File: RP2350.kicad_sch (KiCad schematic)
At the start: 36 parts, among them SW1 SW_Push, SW2 SW_Push, SW3 SW_Push, U1 RP2350A, U4 AMS1117-3.3, U5 ABM8-272-T3_C20625731

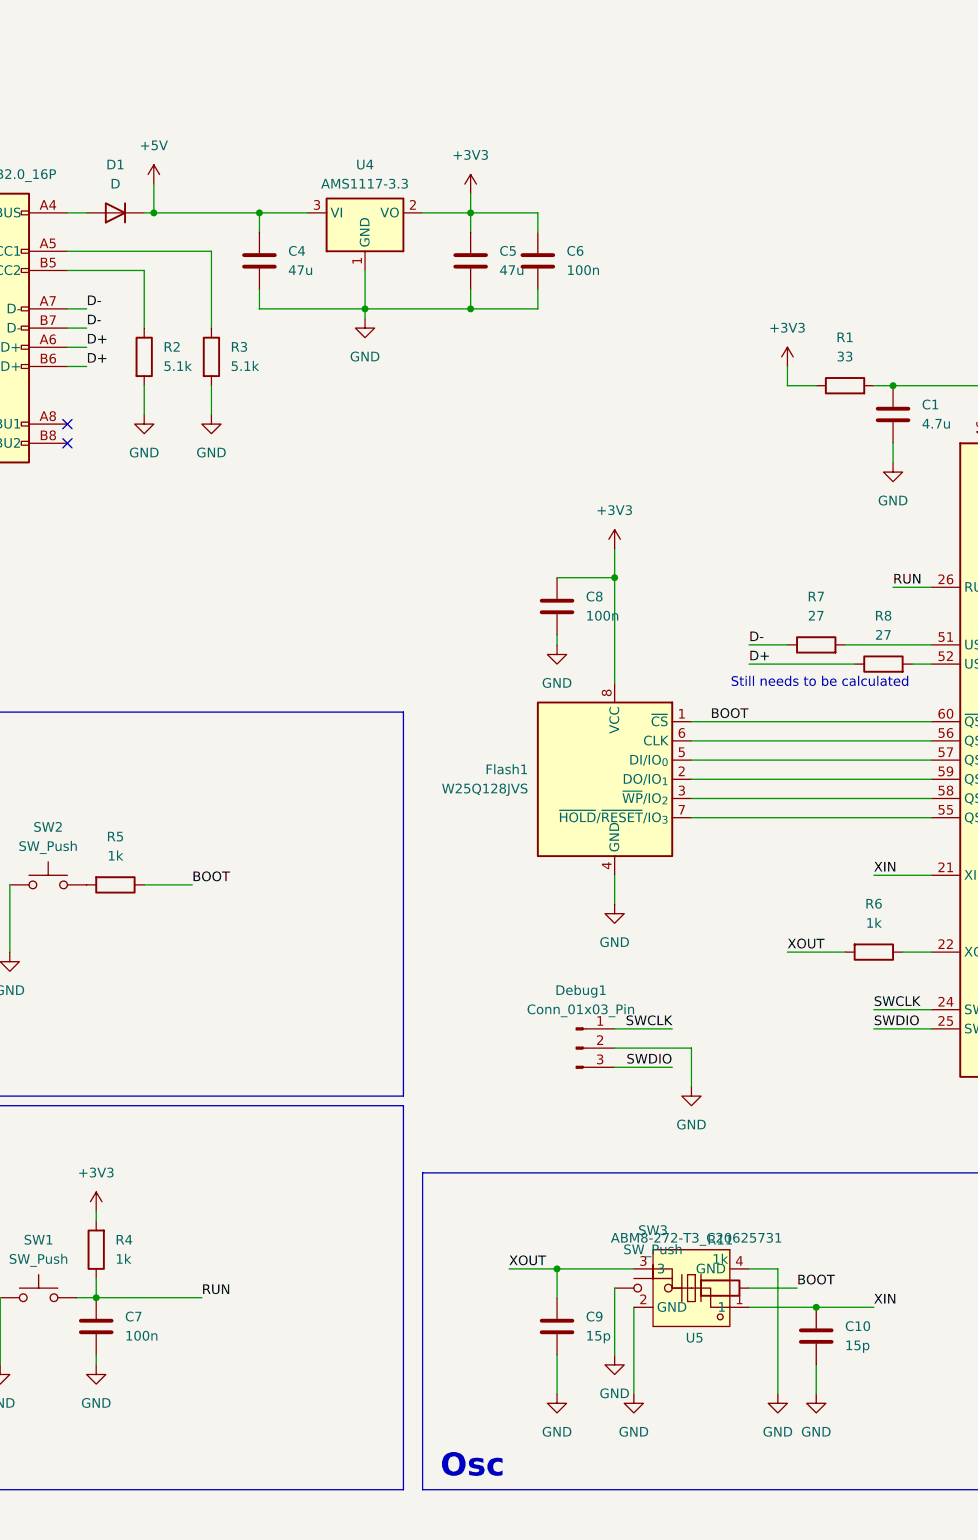
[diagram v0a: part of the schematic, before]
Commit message: generated pdf
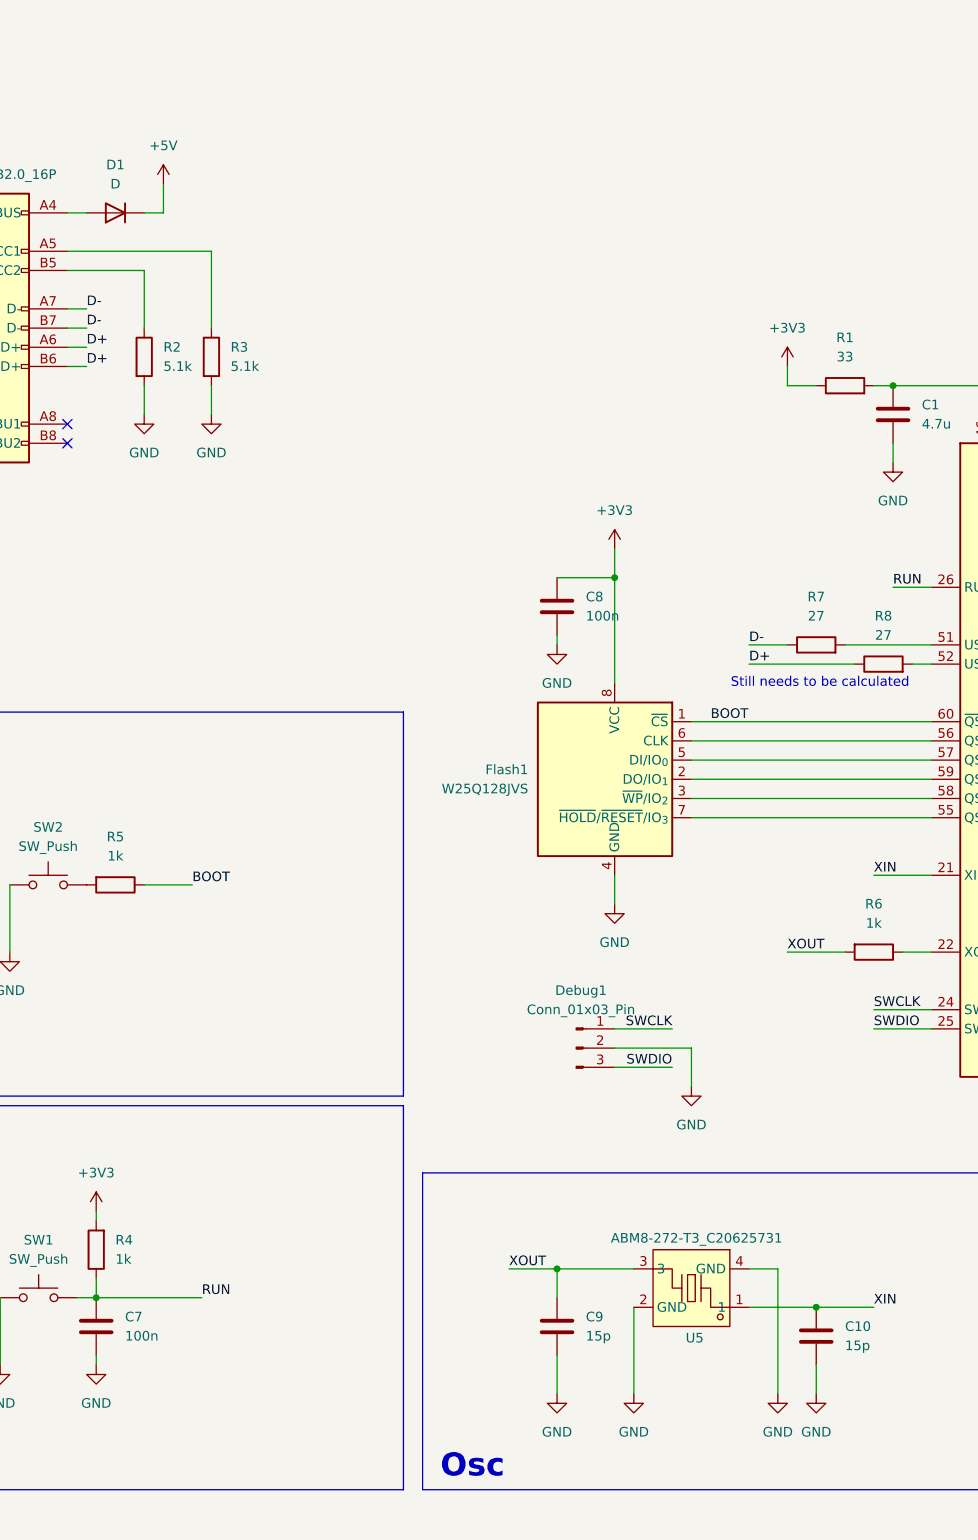
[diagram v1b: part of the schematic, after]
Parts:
- removed C4, C5: 47u, Capacitor_SMD:C_0805_2012Metric_Pad1.18x1.45mm_HandSolder, symbol Device:C
- removed C6: 100n, Capacitor_SMD:C_0805_2012Metric_Pad1.18x1.45mm_HandSolder, symbol Device:C
- removed R11: 1k, Resistor_SMD:R_0805_2012Metric_Pad1.20x1.40mm_HandSolder, symbol Device:R
- removed SW3: SW_Push, Button_Switch_SMD:SW_SPST_EVQPE1, symbol Switch:SW_Push
- removed U4: AMS1117-3.3, Package_TO_SOT_SMD:SOT-223-3_TabPin2, symbol Regulator_Linear:AMS1117-3.3
